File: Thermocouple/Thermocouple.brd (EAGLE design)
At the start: 25.4 x 25.4 mm, 20 parts, among them Q2 BSS138

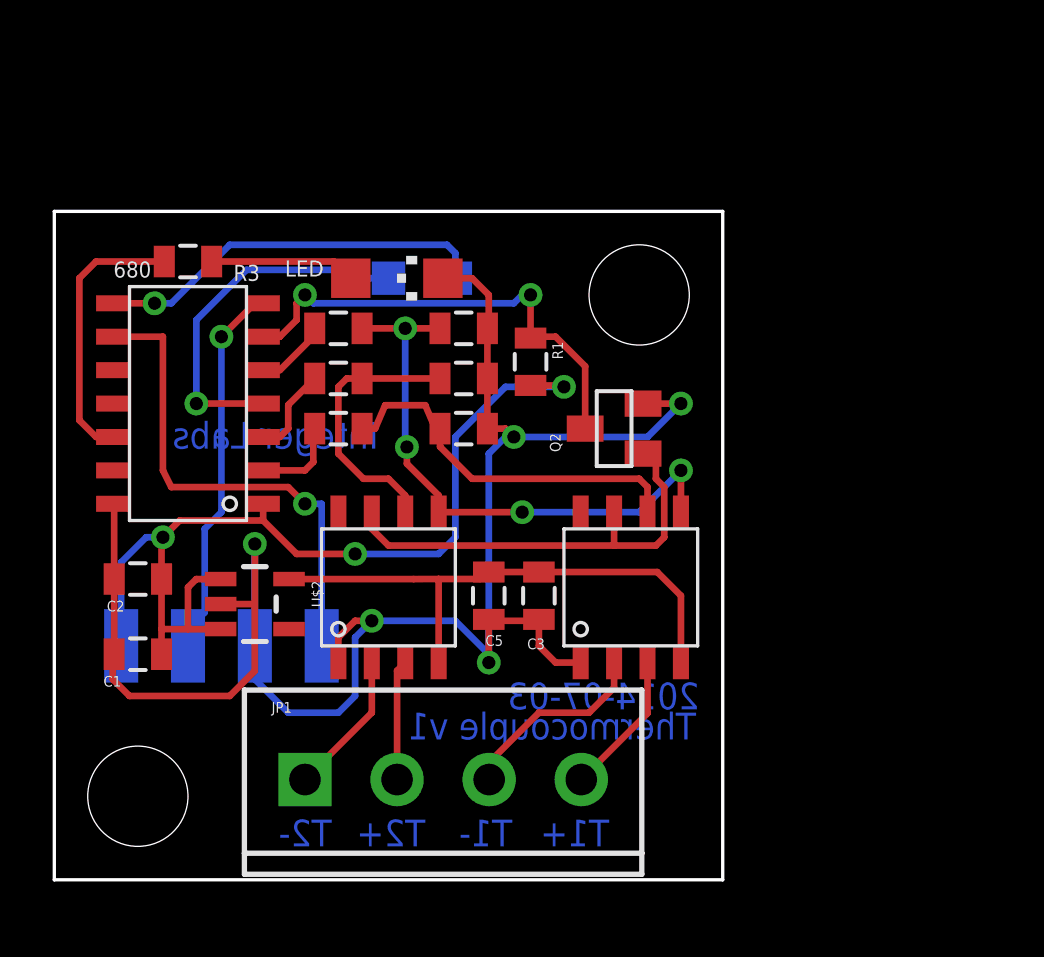
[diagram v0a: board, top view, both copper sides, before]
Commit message: Latest version of schematics and boards
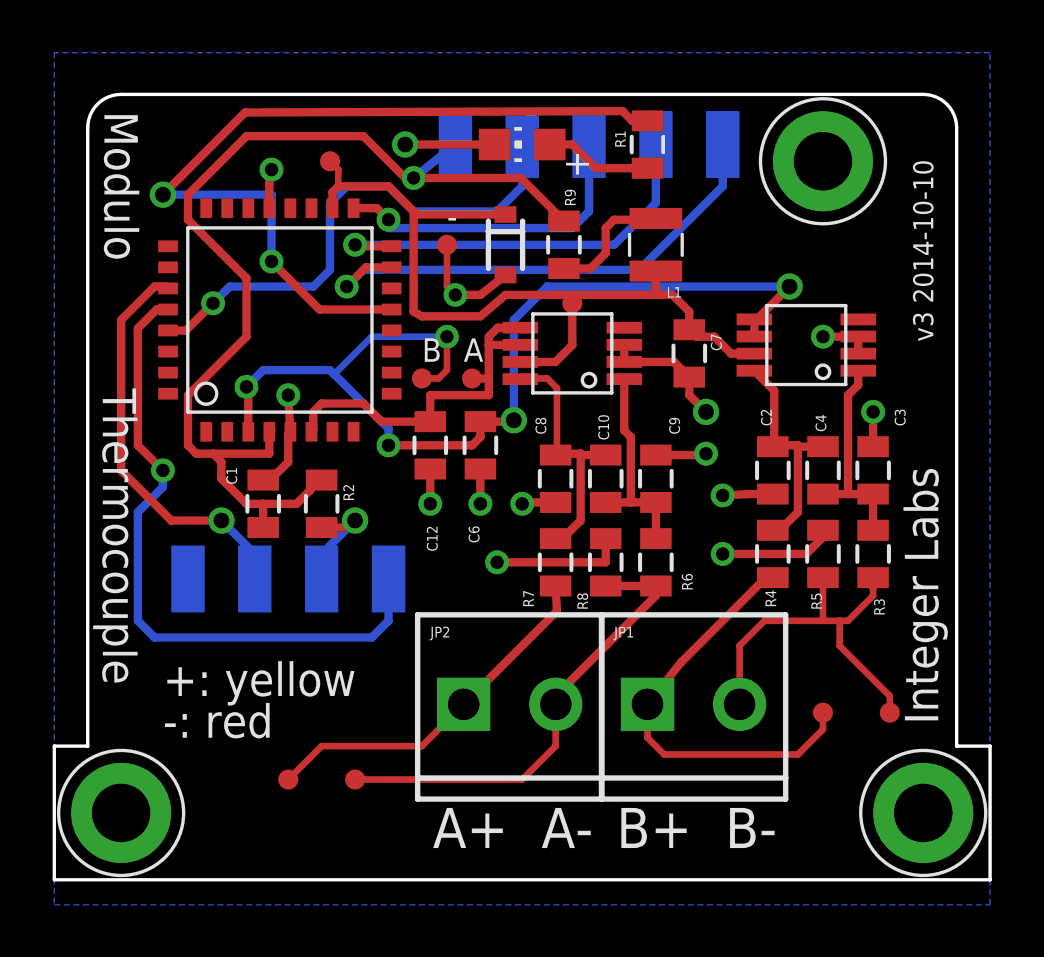
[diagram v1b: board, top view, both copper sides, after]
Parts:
- removed C5: 10uF, SparkFun-Capacitors:0805
- removed LED: blue, led:CHIPLED_1206
- removed Q2: BSS138, SparkFun-DiscreteSemi:SOT23
- added C10, C4: 1uF, SparkFun-Capacitors:0805
- added C12, C6, C8, C9: .1uF, SparkFun-Capacitors:0805
- added C7: .47uF, SparkFun-Capacitors:0805
- added JP2: M023.5MM, SparkFun-Connectors:SCREWTERMINAL-3.5MM-2
- added L1: 1mH, SparkFun-Passives:1007
- added LED1: (no value), adafruit:CHIP-LED0805
- added R4: 24k, SparkFun-Resistors:0805
- added TP1, TP2, TP3, TP4, TP5, TP6, TP7, TP8, TP9: TEST-POINT3, SparkFun-Passives:PAD.03X.03
- C1: value .1uF -> .47uF
- C2: value 10uF -> .1uF
- JP1: value (none) -> M023.5MM; device SparkFun-Connectors:SCREWTERMINAL-3.5MM-4 -> SparkFun-Connectors:SCREWTERMINAL-3.5MM-2
- R1: value 1k -> 680; device SparkFun-Resistors:0805 -> SparkFun-Passives:0805
- R2: value 2k -> 1
- R3: value 680 -> 24k; device SparkFun-Passives:0805 -> SparkFun-Resistors:0805
- R5, R8: value 1k -> 1M
- R6: value 2k -> 24k
- R7: value 1k -> 24k
- R9: value 2k -> 22; device SparkFun-Resistors:0805 -> SparkFun-Passives:0805
- U$1: value MAX31855 -> AD8495; device IntegerLabs:SOIC-8 -> IntegerLabs:MSOP-8
- U$2: value MIC5205-3.3 -> FOOTPRINTFOOTPRINT-2; device SparkFun-PowerIC:SOT23-5 -> IntegerLabs:FOOTPRINT2
- U$3: value TINY841 -> ATTINY48/88-TQFP; device IntegerLabs:SOIC14 -> IntegerLabs:TQFP-32
- U$4: value FOOTPRINT -> AD8495; device IntegerLabs:FOOTPRINT -> IntegerLabs:MSOP-8
- U$5: value MAX31855 -> zener; device IntegerLabs:SOIC-8 -> SparkFun-DiscreteSemi:SOD-323
- moved R3 28.3 mm to (31.1, 12.4), turned to 90 degrees
- moved U$4 28.1 mm to (19.7, 20.0), turned to 90 degrees
- moved C2 24.5 mm to (27.3, 15.6), turned to 270 degrees
- moved R5 14.5 mm to (29.2, 12.4), turned to 270 degrees
- moved R6 13.9 mm to (22.9, 12.1), turned to 90 degrees
- moved U$5 13.7 mm to (17.1, 24.1), turned to 270 degrees
- moved C3 13.6 mm to (31.1, 15.6)
- moved JP1 13.3 mm to (22.5, 6.67)
- moved U$2 13.0 mm to (0.00, 0.00), turned to 0 degrees
- moved U$1 11.5 mm to (28.6, 20.3), turned to 90 degrees
- moved R8 10.4 mm to (21.0, 12.1), turned to 270 degrees
- moved R1 9.38 mm to (22.5, 27.9), turned to 90 degrees
- moved R9 9.14 mm to (19.4, 24.1), turned to 90 degrees
- moved U$3 7.96 mm to (8.57, 21.3)
- moved R7 7.81 mm to (19.1, 12.1), turned to 90 degrees
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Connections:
- removed net +3.3V: C3.1, C5.1, U$1.4, U$2.5, U$5.4
- removed net +5V: C1.1, C2.1, R1.2, U$2.1, U$2.3, U$3.1, U$4.P$1
- removed net CS1: R2.2, U$3.2
- removed net CS1-3.3: R2.1, R5.2, U$1.6
- removed net CS2: R6.2, U$3.3
- removed net CS2-3.3: R6.1, R7.2, U$5.6
- removed net MISO3.3: Q2.1, U$1.7, U$5.7
- removed net MISO5: Q2.3, R1.1, U$3.6
- removed net SCK-3.3: R8.2, R9.1, U$1.5, U$5.5
- removed net SCL/SCK: U$3.9, U$4.P$4
- removed net SDA/MOSI: U$3.7, U$4.P$2
- removed net T1+: JP1.4, U$1.3
- removed net T1-: JP1.3, U$1.2
- removed net T2+: JP1.2, U$5.3
- removed net T2-: JP1.1, U$5.2
- new net AVCC: C7.1, L1.1, TP4.P$1, TP5.P$1, U$1.7, U$3.18, U$4.7, U$5.1
- new net IN1+: JP1.1, R4.1, TP6.P$1
- new net IN1-: JP1.2, R3.1, R5.2, TP7.P$1
- new net IN2+: JP2.1, R7.1, TP8.P$1
- new net IN2-: JP2.2, R6.1, R8.2, TP9.P$1
- new net MOSI: U$2.PROG4, U$3.15
- new net N$2: R2.2, U$2.BUS2
- new net N$3: C3.2, C4.1, R3.2, U$1.1
- new net N$4: C2.1, C4.2, R4.2, U$1.8
- new net N$6: C10.2, C8.1, R7.2, U$4.8
- new net N$7: L1.2, R9.1
- new net N$8: LED1.A, R1.1
- new net SCL: U$2.BUS3, U$3.28
- new net SDA: U$2.BUS1, U$3.27
- new net TEMP1: C6.1, TP1.P$1, U$1.5, U$1.6, U$3.3
- new net TEMP2: C12.1, TP2.P$1, U$3.6, U$4.5, U$4.6
- new net VCC: C1.2, R2.1, R9.2, U$2.PROG0, U$3.4
- net GND: now also C1.1, C12.2, C3.1, C6.2, C7.2, C8.2, C9.1, LED1.C, TP3.P$1, U$1.2, U$1.3, U$2.BUS0, U$3.21, U$3.5, U$4.2, U$4.3, U$5.2; no longer C1.2, C3.2, C5.2, LED.C, Q2.2, R7.1, U$1.1, U$2.2, U$3.14, U$4.P$3, U$5.1
- net LED: now also R1.2, U$3.13; no longer R3.2, U$3.12
- net MISO: now also U$2.PROG3, U$3.16; no longer U$3.8, U$4.MISO
- net N$5: now also C10.1, C9.2, R6.2, U$4.1; no longer LED.A, R3.1
- net RESET: now also U$2.PROG1, U$3.29; no longer U$3.4, U$4.RESET
- net SCK: now also U$2.PROG2, U$3.17; no longer R9.2, U$3.5
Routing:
- net VCC: track 0.00 -> 40.9 mm, vias 0 -> 1
- net TEMP1: track 0.00 -> 39.0 mm, vias 0 -> 5
- net +5V: track 37.7 -> 0.00 mm, vias 3 -> 0
- net GND: track 72.3 -> 38.8 mm, vias 5 -> 14
- net AVCC: track 0.00 -> 32.3 mm
- net SCL: track 0.00 -> 25.0 mm, vias 0 -> 1
- net SCK-3.3: track 21.9 -> 0.00 mm, vias 4 -> 0
- net LED: track 10.4 -> 31.9 mm, vias 0 -> 2
- net +3.3V: track 21.2 -> 0.00 mm
- net MOSI: track 0.00 -> 19.5 mm, vias 0 -> 1
- net SCL/SCK: track 19.1 -> 0.00 mm, vias 1 -> 0
- net MISO5: track 18.0 -> 0.00 mm, vias 2 -> 0
- net IN2-: track 0.00 -> 17.9 mm
- net MISO3.3: track 17.2 -> 0.00 mm
- net IN1+: track 0.00 -> 16.1 mm
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- added copper zone on layer 16, net GND
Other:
- board size 25.4 x 25.4 mm -> 35.6 x 29.8 mm
- board text added: "+: yellow"
- board text added: "-"
- board text added: "-: red"
- board text added: "A"
- board text added: "A+"
- board text added: "A-"
- board text added: "B"
- board text added: "B+"
- board text added: "B-"
- board text added: "Modulo"
- board text added: "Thermocouple"
- board text added: "v3 2014-10-10"
- board text removed: "2014-07-03"
- board text removed: "T1+"
- board text removed: "T1-"
- board text removed: "T2+"
- board text removed: "T2-"
- board text removed: "Thermocouple v1"
